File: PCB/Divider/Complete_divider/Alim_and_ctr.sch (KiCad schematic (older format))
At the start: 34 parts

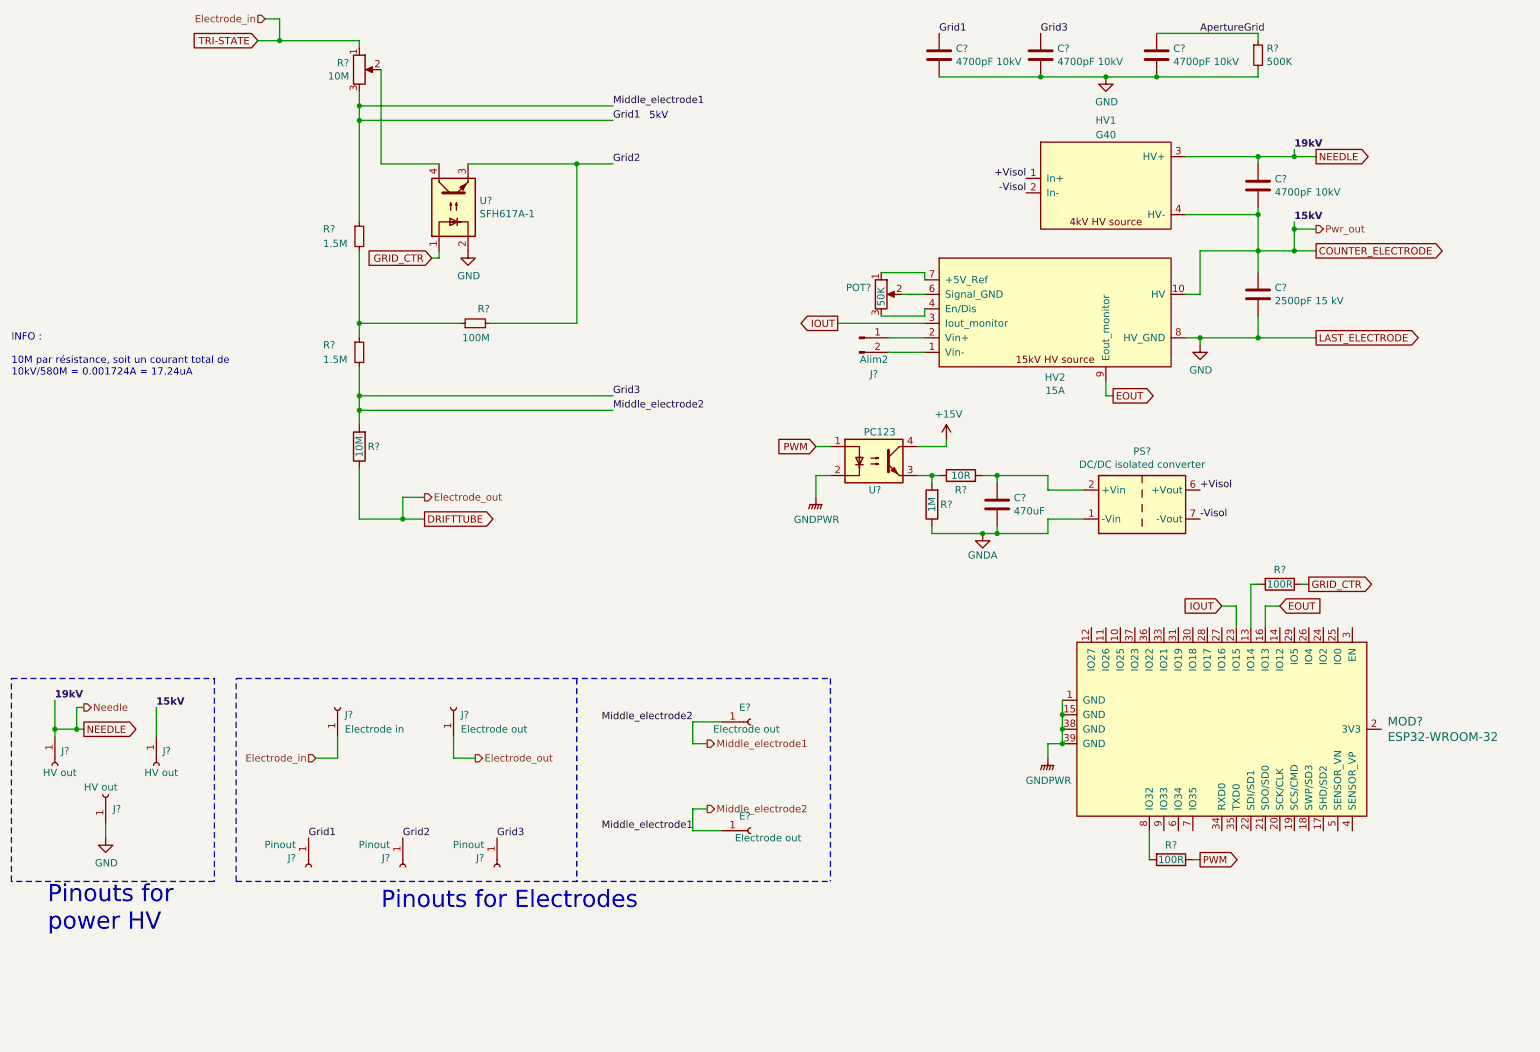
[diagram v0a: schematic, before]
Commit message: Labelling/ordering stuff
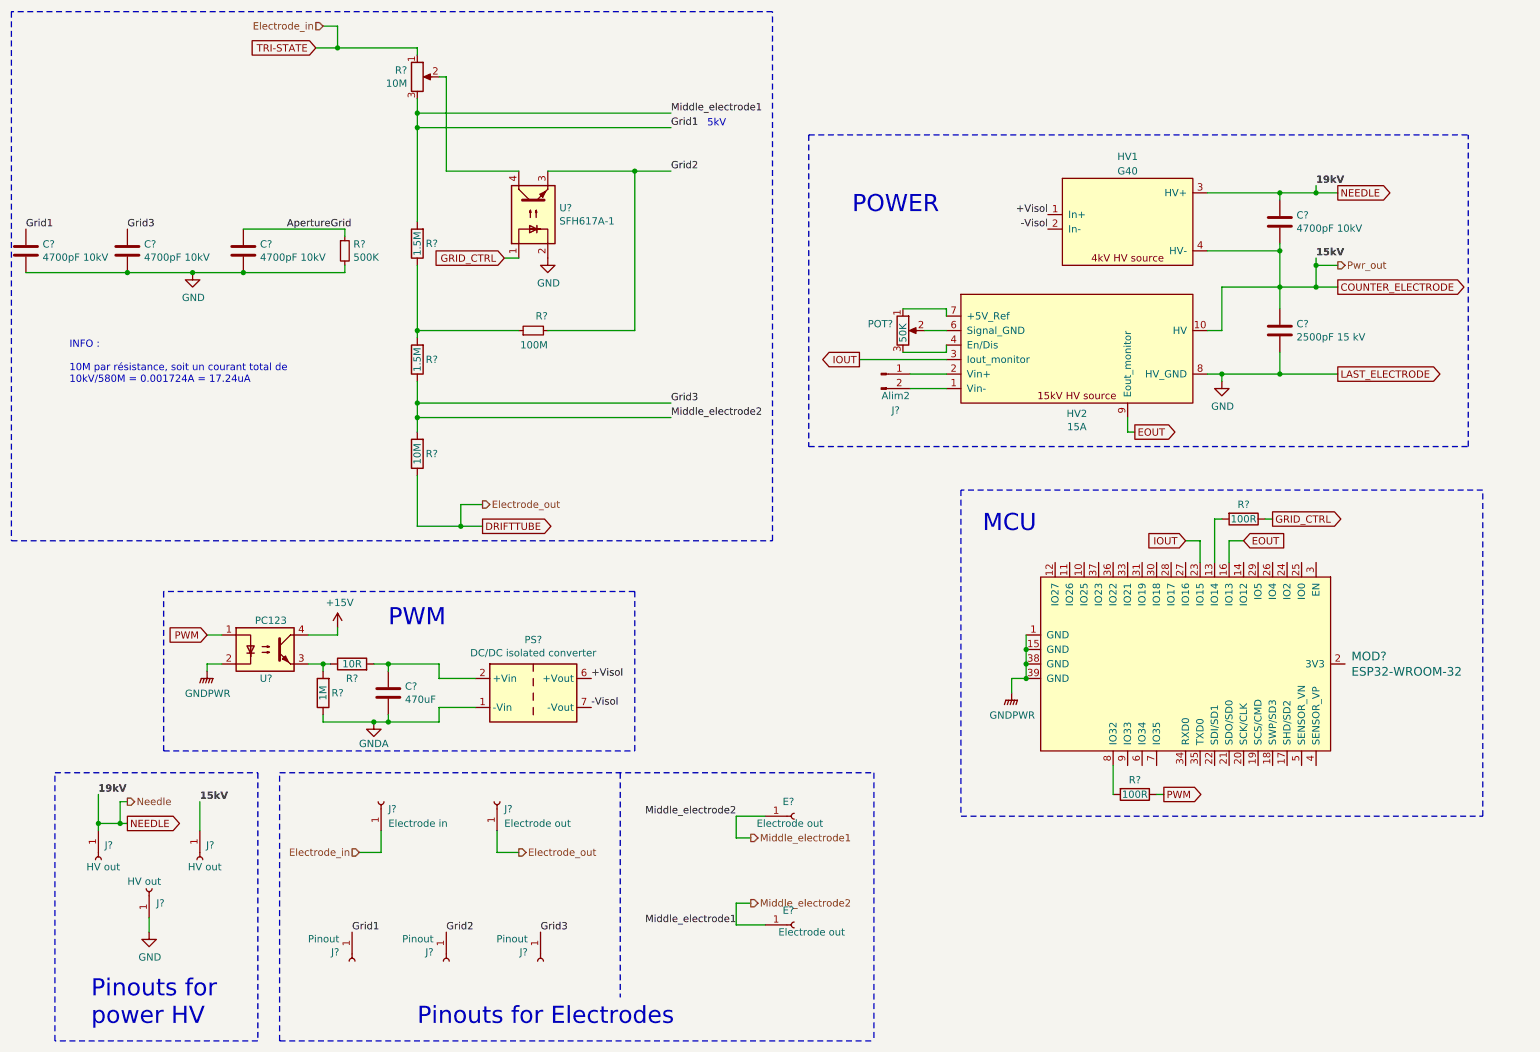
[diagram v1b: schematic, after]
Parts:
- removed R? (x2): 1.5M, Resistor_SMD:R_1206_3216Metric, symbol Device:R_Small
- added R? (x2): 1.5M, symbol Device:R
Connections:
- net Middle_electrode1: now also R?.1, R?.2
- net at R?.1: now also R?.1, R?.2
- net GRID_CTR renamed GRID_CTRL
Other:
- note added: "MCU\n"
- note added: "POWER"
- note added: "PWM \n"
- moved on the sheet: C?, E?, J?, MOD?, POT?, PS?, R?, U?
